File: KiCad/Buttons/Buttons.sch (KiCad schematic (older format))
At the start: 13 parts, among them J1 KEYB, SW1 SET, SW2 OK, SW3 UP, SW4 RHT, SW5 DWN, SW6 LFT

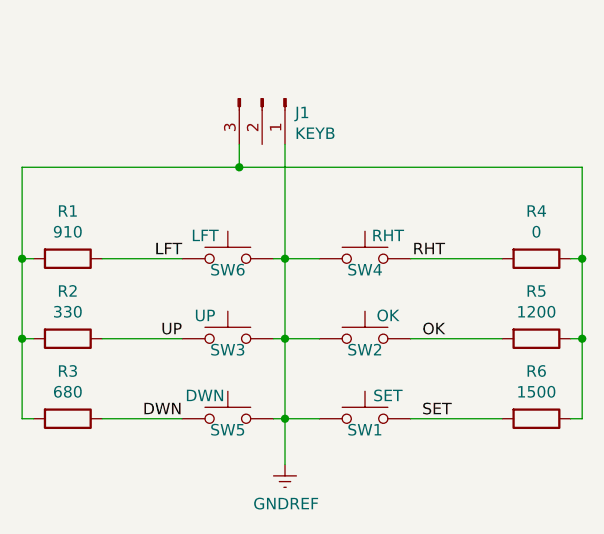
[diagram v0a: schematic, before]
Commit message: ver 2156
Many Updates
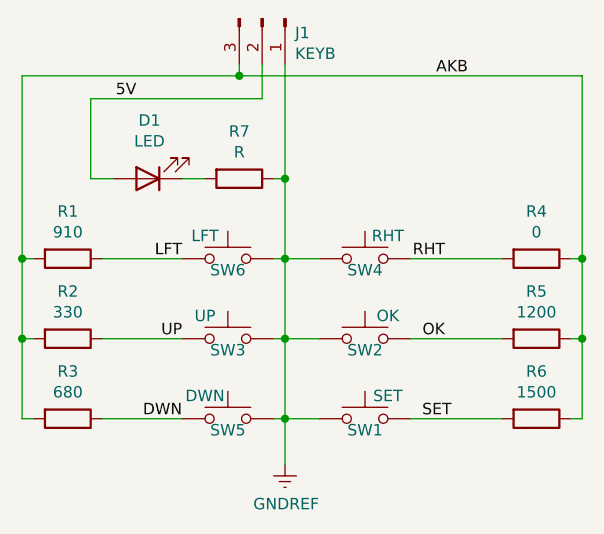
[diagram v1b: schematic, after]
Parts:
- added D1: LED, LED_THT:LED_D3.0mm, symbol Device:LED
- added R7: R, Resistor_SMD:R_0805_2012Metric, symbol Device:R
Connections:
- net GNDREF: now also R7.1
- net AKB: now reaches J1.3 (Pin_3), R1.2, R2.2, R3.2, R4.1, R5.1, R6.1
- net 5V: now reaches J1.2 (Pin_2)
- net 5V: now also D1.2 (A)
- new net: D1.1 (K), R7.2
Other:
- moved on the sheet: J1
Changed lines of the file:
@@
 	5600 3600 6000 3600
-Wire Wire Line
-	5050 2400 5050 2900
-Wire Wire Line
-	3900 2500 3900 2900
 Wire Wire Line
 	3900 3600 3950 3600
@@
 	6300 2900 6350 2900
 Wire Wire Line
-	6350 2900 6350 2500
-Wire Wire Line
 	6350 2900 6350 3250
 Wire Wire Line
@@
 L Connector:Conn_01x03_Male J1
 U 1 1 5F9EC411
-P 4950 2200
-F 0 "J1" V 5012 2344 50  0000 L CNN
-F 1 "KEYB" V 5103 2344 50  0000 L CNN
-F 2 "Connector_PinHeader_2.54mm:PinHeader_1x03_P2.54mm_Vertical" H 4950 2200 50  0001 C CNN
-F 3 "~" H 4950 2200 50  0001 C CNN
-	1    4950 2200
+P 4950 1850
+F 0 "J1" V 5012 1994 50  0000 L CNN
+F 1 "KEYB" V 5103 1994 50  0000 L CNN
+F 2 "Connector_PinHeader_2.54mm:PinHeader_1x03_P2.54mm_Vertical" H 4950 1850 50  0001 C CNN
+F 3 "~" H 4950 1850 50  0001 C CNN
+	1    4950 1850
 	0    1    1    0
 $EndComp
+Text Label 5850 2100 2    50   ~ 0
+AKB
+$Comp
+L Device:R R7
+U 1 1 60388507
+P 4850 2550
+F 0 "R7" V 4643 2550 50  0000 C CNN
+F 1 "R" V 4734 2550 50  0000 C CNN
+F 2 "Resistor_SMD:R_0805_2012Metric" V 4780 2550 50  0001 C CNN
+F 3 "~" H 4850 2550 50  0001 C CNN
+	1    4850 2550
+	0    1    1    0
+$EndComp
+$Comp
+L Device:LED D1
+U 1 1 60388FC9
+P 4450 2550
+F 0 "D1" H 4443 2295 50  0000 C CNN
+F 1 "LED" H 4443 2386 50  0000 C CNN
+F 2 "LED_THT:LED_D3.0mm" H 4450 2550 50  0001 C CNN
+F 3 "~" H 4450 2550 50  0001 C CNN
+	1    4450 2550
+	-1   0    0    1
+$EndComp
 Wire Wire Line
-	3900 2500 4850 2500
+	5050 2050 5050 2550
 Wire Wire Line
-	4850 2400 4850 2500
-Connection ~ 4850 2500
+	4950 2050 4950 2200
 Wire Wire Line
-	4850 2500 6350 2500
+	4950 2200 4200 2200
+Wire Wire Line
+	4200 2200 4200 2550
+Wire Wire Line
+	4200 2550 4300 2550
+Wire Wire Line
+	4600 2550 4700 2550
+Wire Wire Line
+	5000 2550 5050 2550
+Connection ~ 5050 2550
+Wire Wire Line
+	5050 2550 5050 2900
+Wire Wire Line
+	4850 2050 4850 2100
+Wire Wire Line
+	4850 2100 3900 2100
+Wire Wire Line
+	3900 2100 3900 2900
+Wire Wire Line
+	6350 2100 4850 2100
+Wire Wire Line
+	6350 2100 6350 2900
+Connection ~ 4850 2100
+Text Label 4400 2200 2    50   ~ 0
+5V
 $EndSCHEMATC
